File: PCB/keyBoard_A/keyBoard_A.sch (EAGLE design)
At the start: 249 parts, among them IC1 74HC04N, J1 J, J10 J, J11 J, J12 J, J13 J, J14 J, J15 J, J16 J, J17 J, J18 J, J19 J, J2 J, J20 J, J21 J, J22 J, J23 J, J24 J, J25 J, J26 J, J27 J, J28 J, J29 J, J3 J, J30 J, J31 J, J32 J, J33 J, J34 J, J35 J, J36 J, J37 J, J38 J, J39 J, J4 J, J40 J, J41 J, J42 J, J43 J, J44 J, J45 J, J5 J, J6 J, J7 J, J8 J, J9 J

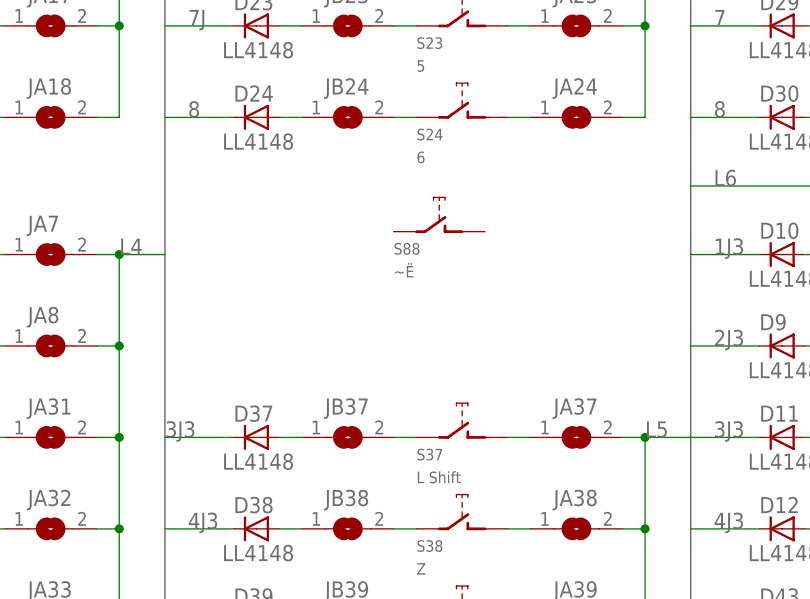
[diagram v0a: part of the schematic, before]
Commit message: pcb b
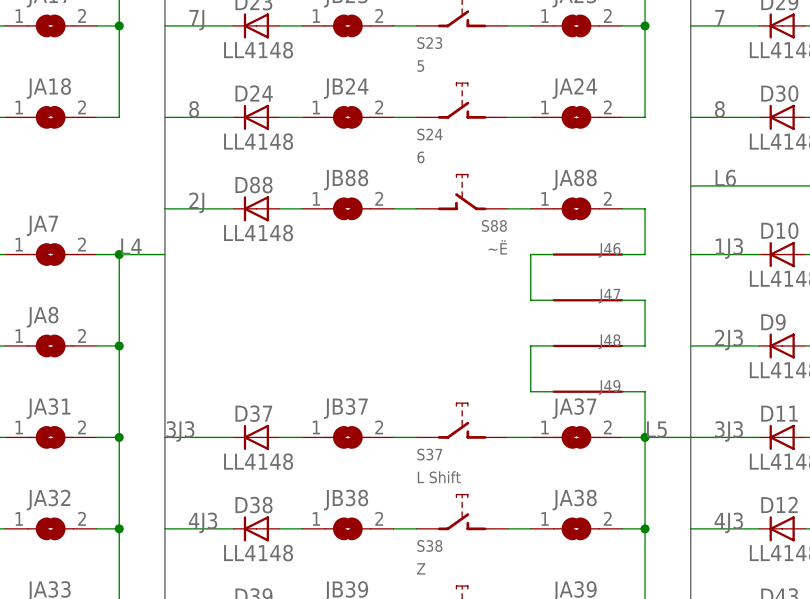
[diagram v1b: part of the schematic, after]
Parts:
- added D88: LL4148, detali:LL4148
- added J46, J47, J48, J49: J, detali_main:J
- added JA88, JB88: (no value), detali:SJ
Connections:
- new net N$117: JB88.2, S88G$1.PIN-2
- new net N$151: D88.A, JB88.1
- new net N$197: JA88.1, S88G$1.PIN-1
- new net N$225: J46.P$1, JA88.2
- new net N$229: J46.P$2, J47.P$2
- new net N$230: J47.P$1, J48.P$1
- new net N$233: J48.P$2, J49.P$2
- net 2J: now also D88.C
- net L5: now also J49.P$1
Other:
- moved on the sheet: S88
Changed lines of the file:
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@@
 <part name="S44A" library="cherrymx" deviceset="CHERRY-MX" device="" value="Fn1"/>
 <part name="S88" library="cherrymx" deviceset="CHERRY-MX-4P" device="" value="~Ё"/>
+<part name="JA88" library="detali" deviceset="SJ" device=""/>
+<part name="JB88" library="detali" deviceset="SJ" device=""/>
+<part name="D88" library="detali" deviceset="LL4148" device=""/>
+<part name="J46" library="detali_main" deviceset="J" device=""/>
+<part name="J47" library="detali_main" deviceset="J" device=""/>
+<part name="J48" library="detali_main" deviceset="J" device=""/>
+<part name="J49" library="detali_main" deviceset="J" device=""/>
 </parts>
 <sheets>
@@
 </instance>
 <instance part="S44A" gate="G$1" x="238.76" y="152.4"/>
-<instance part="S88" gate="G$1" x="127" y="205.74"/>
+<instance part="S88" gate="G$1" x="129.54" y="208.28" rot="MR0"/>
+<instance part="JA88" gate="1" x="142.24" y="208.28"/>
+<instance part="JB88" gate="1" x="116.84" y="208.28"/>
+<instance part="D88" gate="G$1" x="106.68" y="208.28"/>
+<instance part="J46" gate="G$1" x="142.24" y="203.2" smashed="yes">
+<attribute name="NAME" x="144.78" y="203.2" size="1.27" layer="95"/>
+</instance>
+<instance part="J47" gate="G$1" x="142.24" y="198.12" smashed="yes">
+<attribute name="NAME" x="144.78" y="198.12" size="1.27" layer="95"/>
+</instance>
+<instance part="J48" gate="G$1" x="142.24" y="193.04" smashed="yes">
+<attribute name="NAME" x="144.78" y="193.04" size="1.27" layer="95"/>
+</instance>
+<instance part="J49" gate="G$1" x="142.24" y="187.96" smashed="yes">
+<attribute name="NAME" x="144.78" y="187.96" size="1.27" layer="95"/>
+</instance>
 </instances>
 <busses>
@@
 <wire x1="177.8" y1="114.3" x2="182.88" y2="114.3" width="0.1524" layer="91"/>
 <label x="180.34" y="114.3" size="1.778" layer="95"/>
+</segment>
+<segment>
+<pinref part="D88" gate="G$1" pin="C"/>
+<wire x1="96.52" y1="208.28" x2="104.14" y2="208.28" width="0.1524" layer="91"/>
+<label x="99.06" y="208.28" size="1.778" layer="95"/>
 </segment>
 </net>
@@
 <junction x="149.86" y="182.88"/>
 <label x="149.86" y="182.88" size="1.778" layer="95"/>
+<wire x1="149.86" y1="187.96" x2="149.86" y2="182.88" width="0.1524" layer="91"/>
+<pinref part="J49" gate="G$1" pin="P$1"/>
+<wire x1="147.32" y1="187.96" x2="149.86" y2="187.96" width="0.1524" layer="91"/>
 </segment>
 <segment>
@@
 </segment>
 </net>
+<net name="N$151" class="0">
+<segment>
+<pinref part="D88" gate="G$1" pin="A"/>
+<pinref part="JB88" gate="1" pin="1"/>
+<wire x1="109.22" y1="208.28" x2="111.76" y2="208.28" width="0.1524" layer="91"/>
+</segment>
+</net>
+<net name="N$117" class="0">
+<segment>
+<pinref part="JB88" gate="1" pin="2"/>
+<pinref part="S88" gate="G$1" pin="PIN-2"/>
+<wire x1="121.92" y1="208.28" x2="124.46" y2="208.28" width="0.1524" layer="91"/>
+</segment>
+</net>
+<net name="N$197" class="0">
+<segment>
+<pinref part="S88" gate="G$1" pin="PIN-1"/>
+<pinref part="JA88" gate="1" pin="1"/>
+<wire x1="134.62" y1="208.28" x2="137.16" y2="208.28" width="0.1524" layer="91"/>
+</segment>
+</net>
+<net name="N$225" class="0">
+<segment>
+<pinref part="JA88" gate="1" pin="2"/>
+<wire x1="147.32" y1="208.28" x2="149.86" y2="208.28" width="0.1524" layer="91"/>
+<wire x1="149.86" y1="208.28" x2="149.86" y2="203.2" width="0.1524" layer="91"/>
+<pinref part="J46" gate="G$1" pin="P$1"/>
+<wire x1="149.86" y1="203.2" x2="147.32" y2="203.2" width="0.1524" layer="91"/>
+</segment>
+</net>
+<net name="N$229" class="0">
+<segment>
+<pinref part="J46" gate="G$1" pin="P$2"/>
+<wire x1="139.7" y1="203.2" x2="137.16" y2="203.2" width="0.1524" layer="91"/>
+<wire x1="137.16" y1="203.2" x2="137.16" y2="198.12" width="0.1524" layer="91"/>
+<pinref part="J47" gate="G$1" pin="P$2"/>
+<wire x1="137.16" y1="198.12" x2="139.7" y2="198.12" width="0.1524" layer="91"/>
+</segment>
+</net>
+<net name="N$230" class="0">
+<segment>
+<pinref part="J47" gate="G$1" pin="P$1"/>
+<wire x1="147.32" y1="198.12" x2="149.86" y2="198.12" width="0.1524" layer="91"/>
+<wire x1="149.86" y1="198.12" x2="149.86" y2="193.04" width="0.1524" layer="91"/>
+<pinref part="J48" gate="G$1" pin="P$1"/>
+<wire x1="149.86" y1="193.04" x2="147.32" y2="193.04" width="0.1524" layer="91"/>
+</segment>
+</net>
+<net name="N$233" class="0">
+<segment>
+<pinref part="J48" gate="G$1" pin="P$2"/>
+<wire x1="139.7" y1="193.04" x2="137.16" y2="193.04" width="0.1524" layer="91"/>
+<wire x1="137.16" y1="193.04" x2="137.16" y2="187.96" width="0.1524" layer="91"/>
+<pinref part="J49" gate="G$1" pin="P$2"/>
+<wire x1="137.16" y1="187.96" x2="139.7" y2="187.96" width="0.1524" layer="91"/>
+</segment>
+</net>

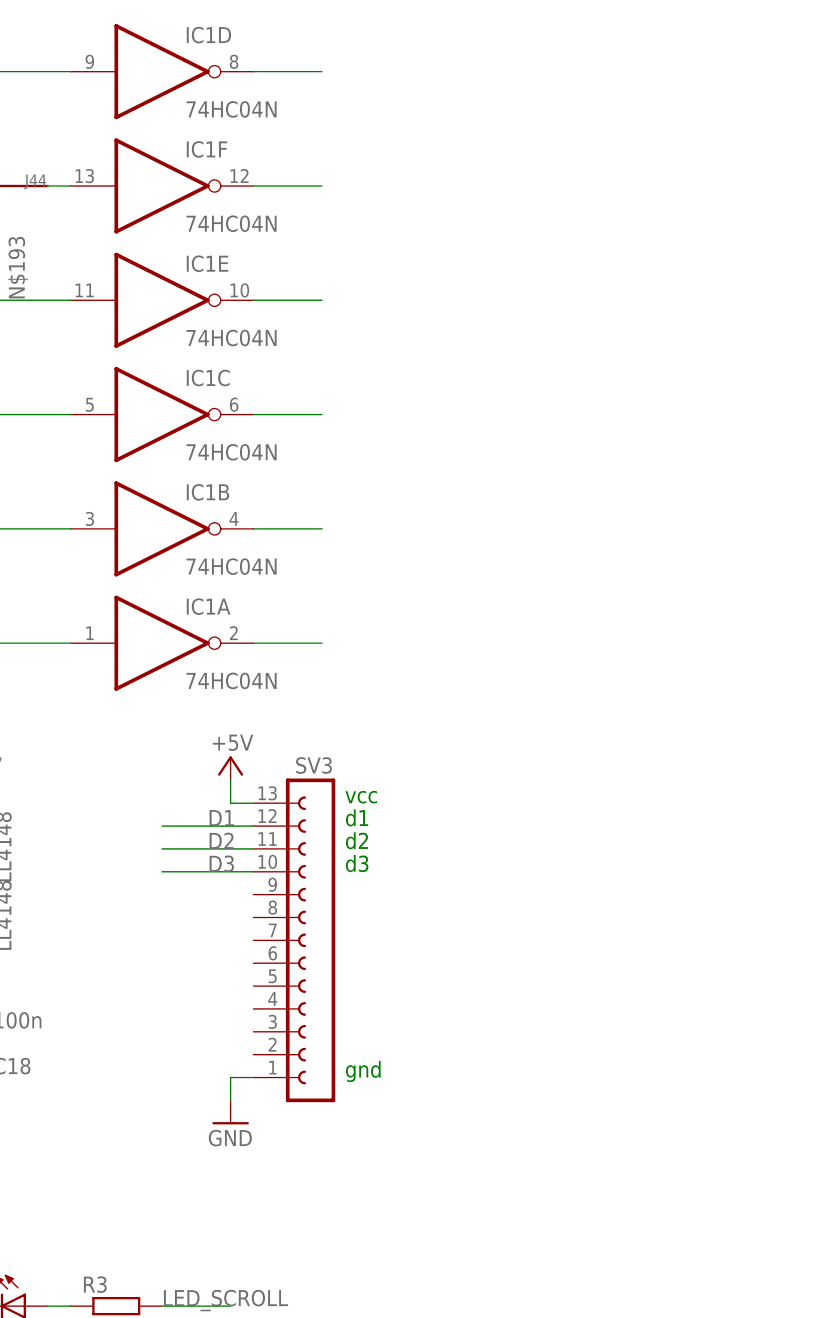
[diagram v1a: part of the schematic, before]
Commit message: .
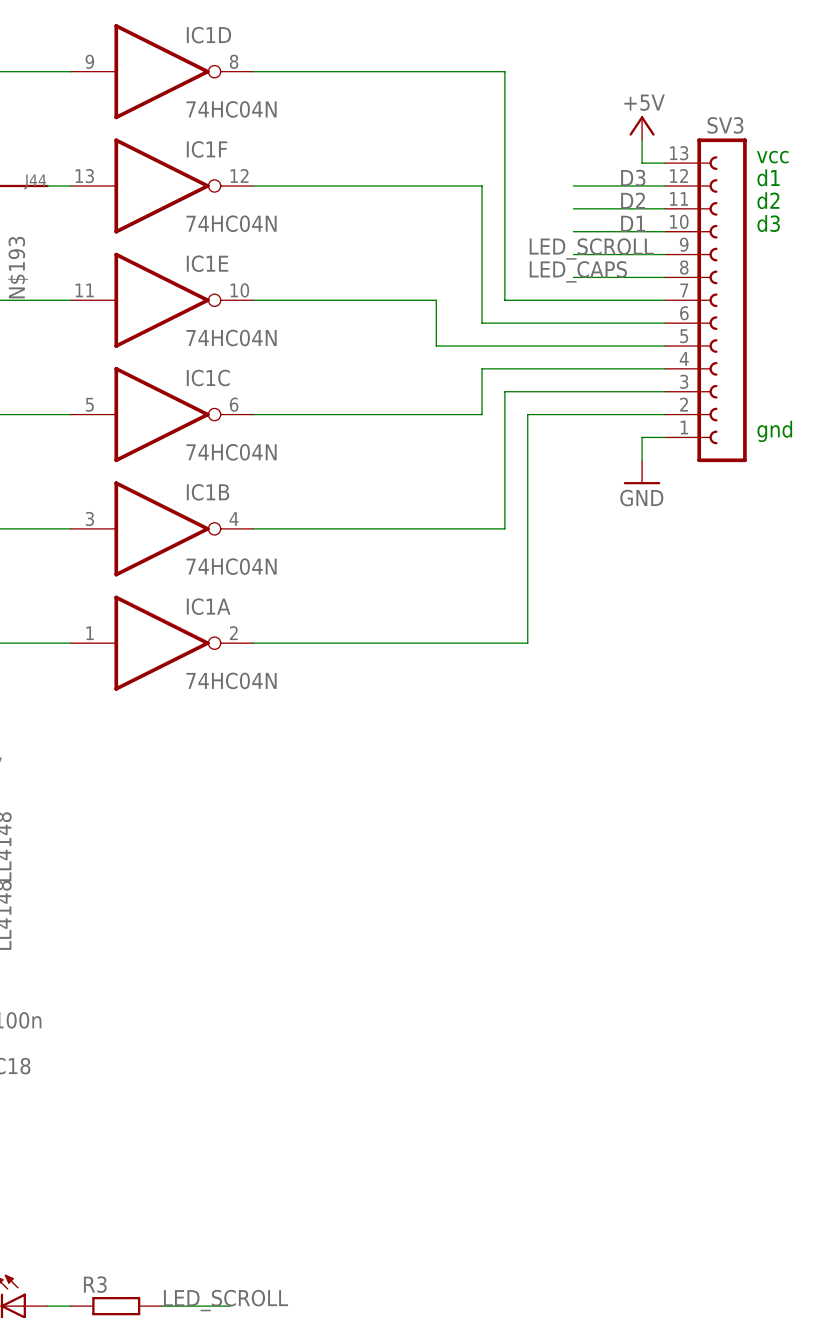
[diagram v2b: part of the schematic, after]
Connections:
- net D1: now also SV3.10; no longer SV3.12
- net D3: now also SV3.12; no longer SV3.10
- net LED_CAPS: now also SV3.8
- net LED_SCROLL: now also SV3.9
- net N$195: now also SV3.6
- net N$196: now also SV3.5
- net N$198: now also SV3.2
- net N$199: now also SV3.3
- net N$200: now also SV3.4
- net N$203: now also SV3.7
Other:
- moved on the sheet: SV3
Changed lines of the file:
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@@
 <description>KB_A</description>
 <plain>
-<text x="322.58" y="251.46" size="1.778" layer="91">d1</text>
-<text x="322.58" y="254" size="1.778" layer="91">vcc</text>
-<text x="322.58" y="248.92" size="1.778" layer="91">d2</text>
-<text x="322.58" y="246.38" size="1.778" layer="91">d3</text>
-<text x="322.58" y="223.52" size="1.778" layer="91">gnd</text>
+<text x="368.3" y="322.58" size="1.778" layer="91">d1</text>
+<text x="368.3" y="325.12" size="1.778" layer="91">vcc</text>
+<text x="368.3" y="320.04" size="1.778" layer="91">d2</text>
+<text x="368.3" y="317.5" size="1.778" layer="91">d3</text>
+<text x="368.3" y="294.64" size="1.778" layer="91">gnd</text>
 <text x="40.64" y="304.8" size="5.08" layer="91">LEFT KB</text>
 </plain>
@@
 <attribute name="NAME" x="279.4" y="309.88" size="1.27" layer="95"/>
 </instance>
-<instance part="SV3" gate="G$1" x="320.04" y="238.76" rot="MR0"/>
-<instance part="GND19" gate="1" x="309.88" y="218.44"/>
-<instance part="P+11" gate="1" x="309.88" y="259.08" smashed="yes">
-<attribute name="VALUE" x="312.42" y="261.62" size="1.778" layer="96" rot="R180"/>
+<instance part="SV3" gate="G$1" x="365.76" y="309.88" rot="MR0"/>
+<instance part="GND19" gate="1" x="355.6" y="289.56"/>
+<instance part="P+11" gate="1" x="355.6" y="330.2" smashed="yes">
+<attribute name="VALUE" x="358.14" y="332.74" size="1.778" layer="96" rot="R180"/>
 </instance>
 <instance part="SCROLL" gate="G$1" x="287.02" y="198.12" rot="R270"/>
@@
 <segment>
 <pinref part="P+11" gate="1" pin="+5V"/>
-<wire x1="309.88" y1="256.54" x2="309.88" y2="254" width="0.1524" layer="91"/>
+<wire x1="355.6" y1="327.66" x2="355.6" y2="325.12" width="0.1524" layer="91"/>
 <pinref part="SV3" gate="G$1" pin="13"/>
-<wire x1="309.88" y1="254" x2="312.42" y2="254" width="0.1524" layer="91"/>
+<wire x1="355.6" y1="325.12" x2="358.14" y2="325.12" width="0.1524" layer="91"/>
 </segment>
 <segment>
@@
 <segment>
 <pinref part="GND19" gate="1" pin="GND"/>
-<wire x1="309.88" y1="220.98" x2="309.88" y2="223.52" width="0.1524" layer="91"/>
+<wire x1="355.6" y1="292.1" x2="355.6" y2="294.64" width="0.1524" layer="91"/>
 <pinref part="SV3" gate="G$1" pin="1"/>
-<wire x1="309.88" y1="223.52" x2="312.42" y2="223.52" width="0.1524" layer="91"/>
+<wire x1="355.6" y1="294.64" x2="358.14" y2="294.64" width="0.1524" layer="91"/>
 </segment>
 </net>
@@
 </segment>
 <segment>
-<pinref part="SV3" gate="G$1" pin="10"/>
-<wire x1="312.42" y1="246.38" x2="302.26" y2="246.38" width="0.1524" layer="91"/>
-<label x="307.34" y="246.38" size="1.778" layer="95"/>
+<pinref part="SV3" gate="G$1" pin="12"/>
+<wire x1="358.14" y1="322.58" x2="347.98" y2="322.58" width="0.1524" layer="91"/>
+<label x="353.06" y="322.58" size="1.778" layer="95"/>
 </segment>
 </net>
@@
 <segment>
 <pinref part="SV3" gate="G$1" pin="11"/>
-<wire x1="312.42" y1="248.92" x2="302.26" y2="248.92" width="0.1524" layer="91"/>
-<label x="307.34" y="248.92" size="1.778" layer="95"/>
+<wire x1="358.14" y1="320.04" x2="347.98" y2="320.04" width="0.1524" layer="91"/>
+<label x="353.06" y="320.04" size="1.778" layer="95"/>
 </segment>
 </net>
@@
 </segment>
 <segment>
-<pinref part="SV3" gate="G$1" pin="12"/>
-<wire x1="312.42" y1="251.46" x2="302.26" y2="251.46" width="0.1524" layer="91"/>
-<label x="307.34" y="251.46" size="1.778" layer="95"/>
+<pinref part="SV3" gate="G$1" pin="10"/>
+<wire x1="358.14" y1="317.5" x2="347.98" y2="317.5" width="0.1524" layer="91"/>
+<label x="353.06" y="317.5" size="1.778" layer="95"/>
 </segment>
 </net>
@@
 <segment>
 <pinref part="IC1" gate="A" pin="O"/>
-<wire x1="312.42" y1="271.78" x2="320.04" y2="271.78" width="0.1524" layer="91"/>
+<wire x1="342.9" y1="297.18" x2="342.9" y2="271.78" width="0.1524" layer="91"/>
+<wire x1="342.9" y1="271.78" x2="312.42" y2="271.78" width="0.1524" layer="91"/>
+<pinref part="SV3" gate="G$1" pin="2"/>
+<wire x1="358.14" y1="297.18" x2="342.9" y2="297.18" width="0.1524" layer="91"/>
 </segment>
 </net>
@@
 <segment>
 <pinref part="IC1" gate="B" pin="O"/>
-<wire x1="312.42" y1="284.48" x2="320.04" y2="284.48" width="0.1524" layer="91"/>
+<wire x1="340.36" y1="299.72" x2="340.36" y2="284.48" width="0.1524" layer="91"/>
+<wire x1="340.36" y1="284.48" x2="312.42" y2="284.48" width="0.1524" layer="91"/>
+<pinref part="SV3" gate="G$1" pin="3"/>
+<wire x1="358.14" y1="299.72" x2="340.36" y2="299.72" width="0.1524" layer="91"/>
 </segment>
 </net>
@@
 <segment>
 <pinref part="IC1" gate="C" pin="O"/>
-<wire x1="312.42" y1="297.18" x2="320.04" y2="297.18" width="0.1524" layer="91"/>
+<wire x1="337.82" y1="302.26" x2="337.82" y2="297.18" width="0.1524" layer="91"/>
+<wire x1="337.82" y1="297.18" x2="312.42" y2="297.18" width="0.1524" layer="91"/>
+<pinref part="SV3" gate="G$1" pin="4"/>
+<wire x1="358.14" y1="302.26" x2="337.82" y2="302.26" width="0.1524" layer="91"/>
 </segment>
 </net>
@@
 <segment>
 <pinref part="IC1" gate="D" pin="O"/>
-<wire x1="312.42" y1="335.28" x2="320.04" y2="335.28" width="0.1524" layer="91"/>
+<wire x1="340.36" y1="309.88" x2="340.36" y2="335.28" width="0.1524" layer="91"/>
+<wire x1="340.36" y1="335.28" x2="312.42" y2="335.28" width="0.1524" layer="91"/>
+<pinref part="SV3" gate="G$1" pin="7"/>
+<wire x1="340.36" y1="309.88" x2="358.14" y2="309.88" width="0.1524" layer="91"/>
 </segment>
 </net>
@@
 <segment>
 <pinref part="IC1" gate="F" pin="O"/>
-<wire x1="312.42" y1="322.58" x2="320.04" y2="322.58" width="0.1524" layer="91"/>
-</segment>
-</net>
-<net name="N$196" class="0">
-<segment>
-<pinref part="IC1" gate="E" pin="O"/>
-<wire x1="312.42" y1="309.88" x2="320.04" y2="309.88" width="0.1524" layer="91"/>
+<wire x1="337.82" y1="307.34" x2="337.82" y2="322.58" width="0.1524" layer="91"/>
+<wire x1="337.82" y1="322.58" x2="312.42" y2="322.58" width="0.1524" layer="91"/>
+<pinref part="SV3" gate="G$1" pin="6"/>
+<wire x1="337.82" y1="307.34" x2="358.14" y2="307.34" width="0.1524" layer="91"/>
 </segment>
 </net>
@@
 <label x="302.26" y="198.12" size="1.778" layer="95"/>
 </segment>
+<segment>
+<pinref part="SV3" gate="G$1" pin="9"/>
+<wire x1="358.14" y1="314.96" x2="347.98" y2="314.96" width="0.1524" layer="91"/>
+<label x="342.9" y="314.96" size="1.778" layer="95"/>
+</segment>
 </net>
 <net name="LED_CAPS" class="0">
@@
 <wire x1="302.26" y1="187.96" x2="309.88" y2="187.96" width="0.1524" layer="91"/>
 <label x="302.26" y="187.96" size="1.778" layer="95"/>
+</segment>
+<segment>
+<pinref part="SV3" gate="G$1" pin="8"/>
+<wire x1="358.14" y1="312.42" x2="347.98" y2="312.42" width="0.1524" layer="91"/>
+<label x="342.9" y="312.42" size="1.778" layer="95"/>
 </segment>
 </net>
@@
 </segment>
 </net>
+<net name="N$196" class="0">
+<segment>
+<pinref part="IC1" gate="E" pin="O"/>
+<wire x1="312.42" y1="309.88" x2="332.74" y2="309.88" width="0.1524" layer="91"/>
+<wire x1="332.74" y1="309.88" x2="332.74" y2="304.8" width="0.1524" layer="91"/>
+<pinref part="SV3" gate="G$1" pin="5"/>
+<wire x1="332.74" y1="304.8" x2="358.14" y2="304.8" width="0.1524" layer="91"/>
+</segment>
+</net>
